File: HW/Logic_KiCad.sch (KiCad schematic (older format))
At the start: 11 parts, among them SW1 SW_SPDT, U1 ESP32-PICO-D4

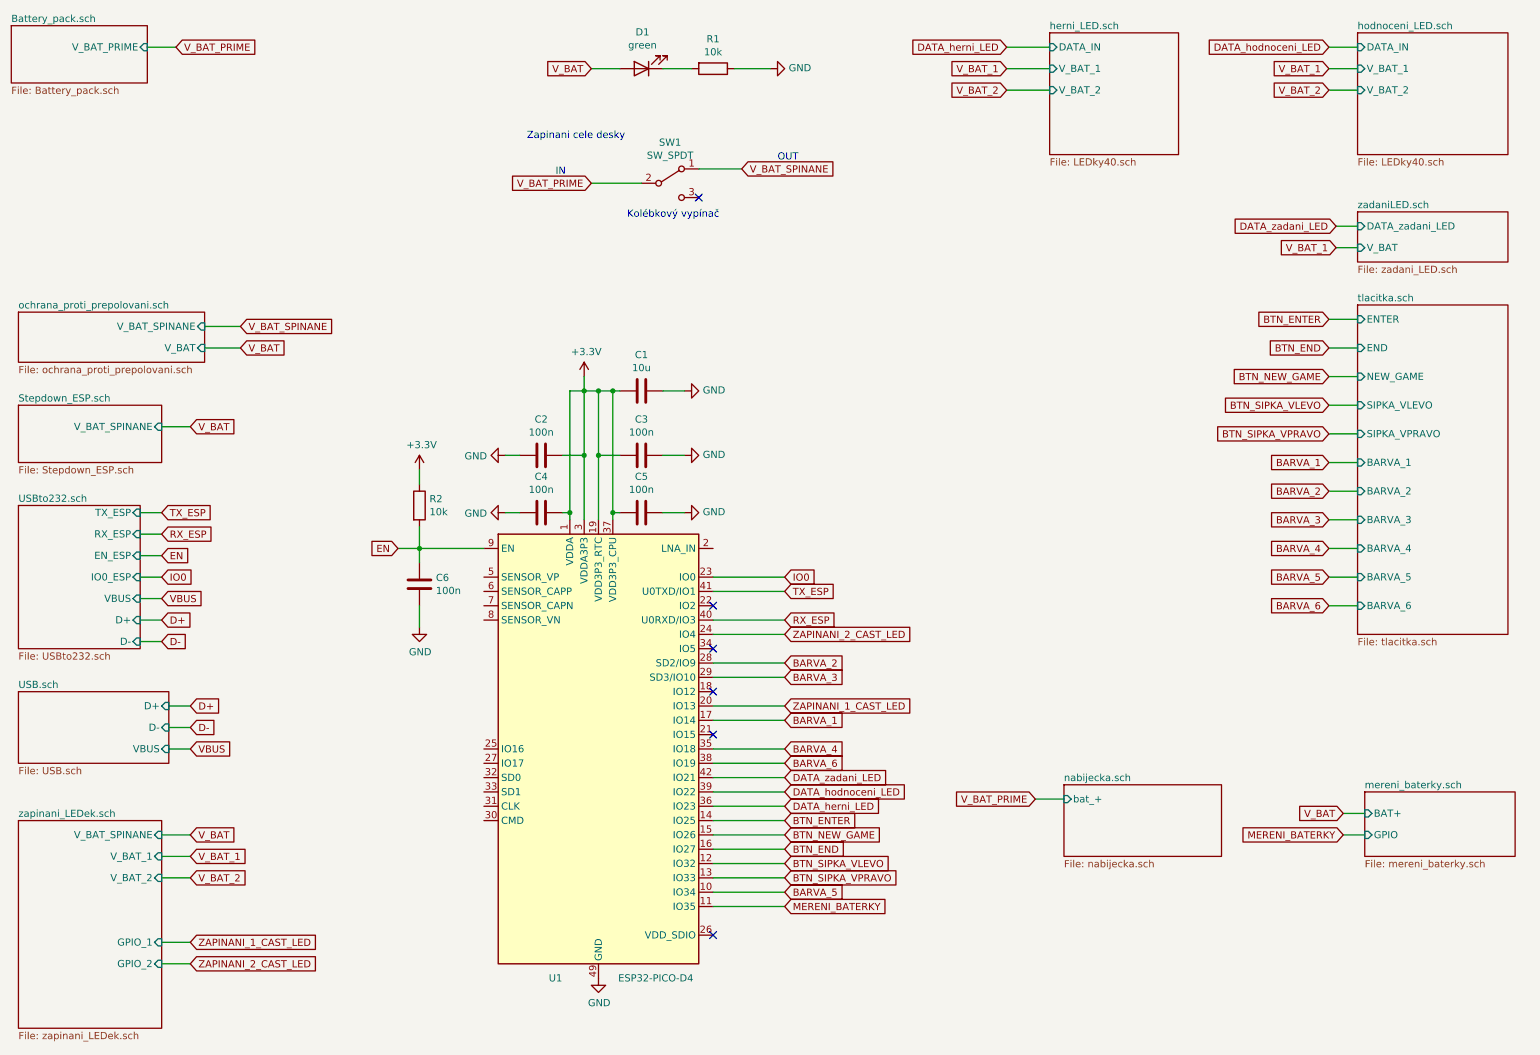
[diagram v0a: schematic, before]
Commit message: deposit of DPS, start v1.0
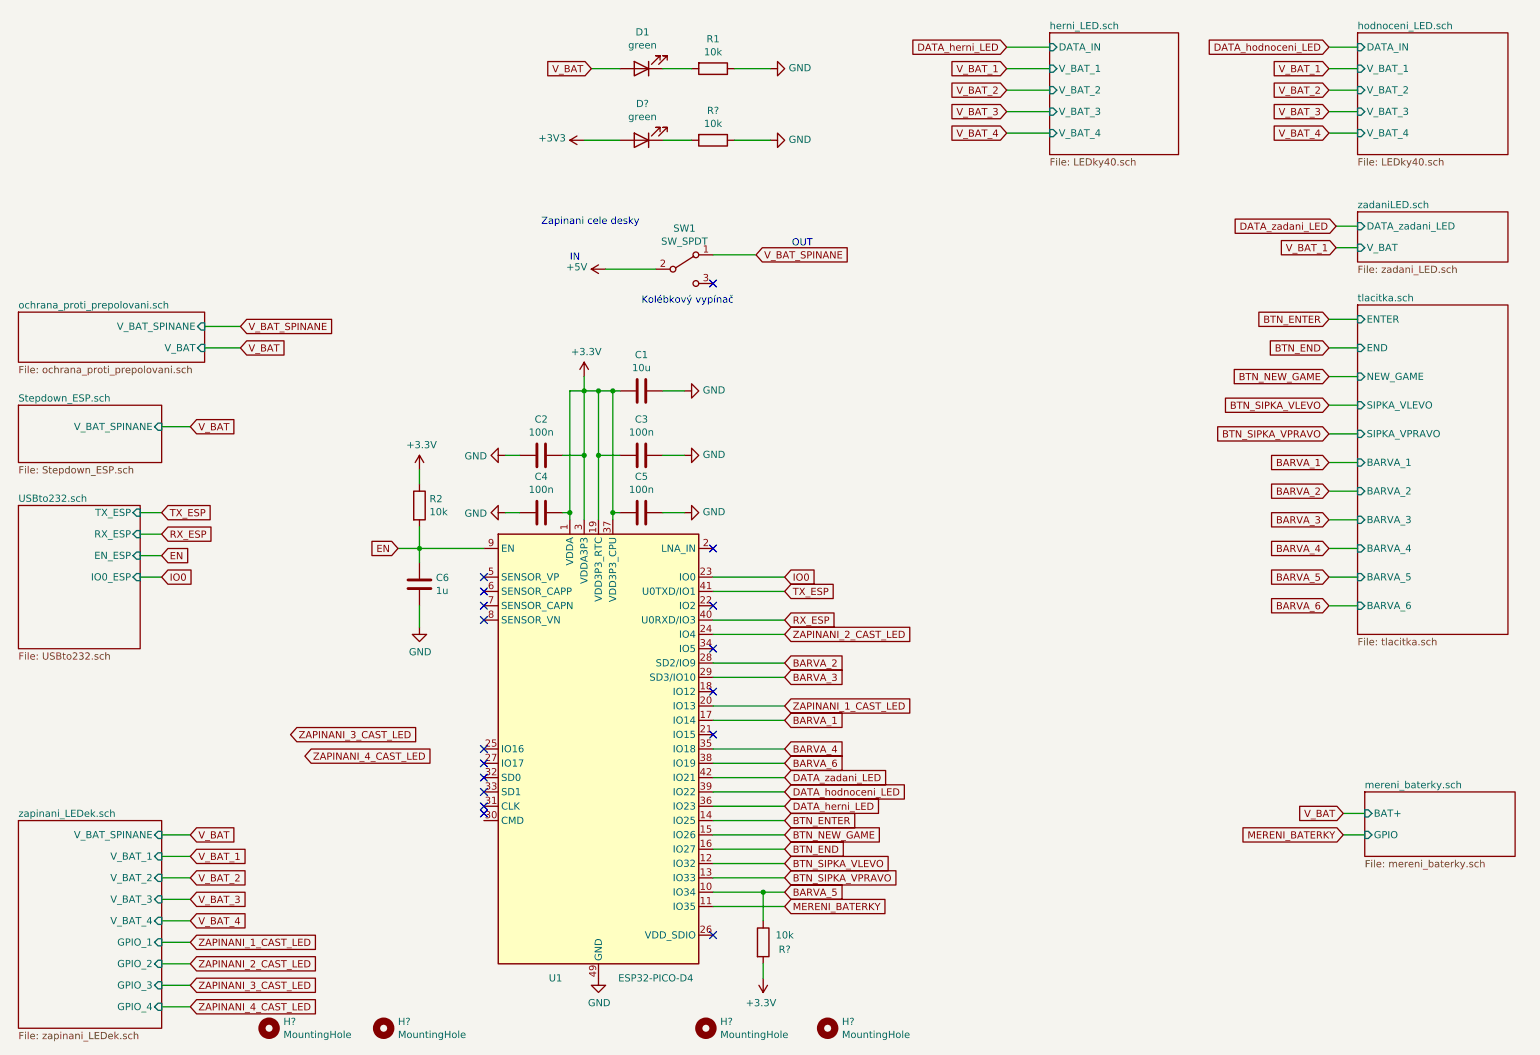
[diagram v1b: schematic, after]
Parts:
- added D?: green, LED_SMD:LED_0603_1608Metric, symbol Device:LED
- added H? (x4): MountingHole, symbol Mechanical:MountingHole
- added R? (x2): 10k, Resistor_SMD:R_0402_1005Metric, symbol Device:R
- C6: value 100n -> 1u; LCSC C1525 -> (none)
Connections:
- net +3V3: now also D?.2 (A), R?.2
- net BARVA_5: now also R?.1
- net GND: now also R?.1
- net V_BAT_PRIME renamed +5V
- new net: D?.1 (K), R?.2
- no-connect marks 6 -> 17
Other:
- moved on the sheet: SW1

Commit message: start place components
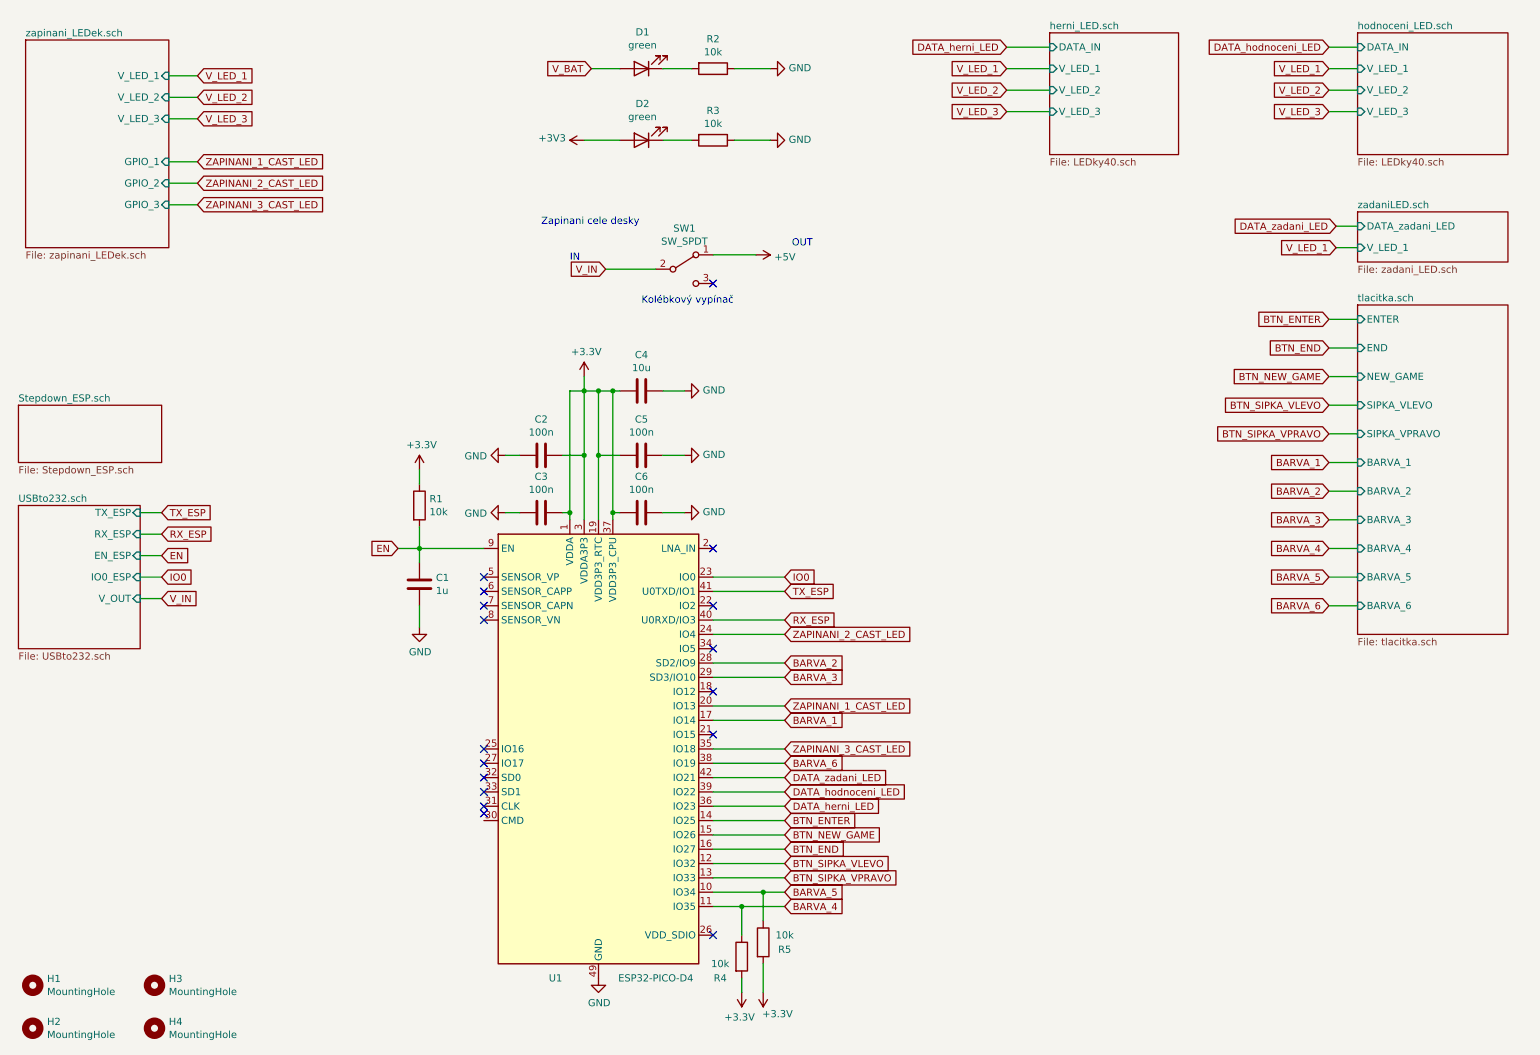
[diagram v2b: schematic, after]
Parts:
- added R4: 10k, Resistor_SMD:R_0402_1005Metric, symbol Device:R
- H1, H2, H3, H4: renamed from H?; footprint (none) -> MountingHole:MountingHole_3.2mm_M3_DIN965_Pad; LCSC (none) -> -
- gave numbers to parts that had none: 3
- renumbered C6 to C1, C4 to C3, C1 to C4, C3 to C5, C5 to C6, R2 to R1, R1 to R2
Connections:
- net MERENI_BATERKY is gone; now on net BARVA_4: U1.11 (IO35)
- net V_BAT_SPINANE is gone; now on net +5V: SW1.1 (A)
- net +3V3: now also R4.2
- net +5V: no longer SW1.2 (B)
- net BARVA_4: now also R4.1; no longer U1.35 (IO18)
- net ZAPINANI_3_CAST_LED: now also U1.35 (IO18)
- new net V_IN: SW1.2 (B)
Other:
- moved on the sheet: H1, H2, H3, H4
